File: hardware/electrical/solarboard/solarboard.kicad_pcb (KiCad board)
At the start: 2 copper layers, 10 parts, among them J1 Conn_01x02_Pin

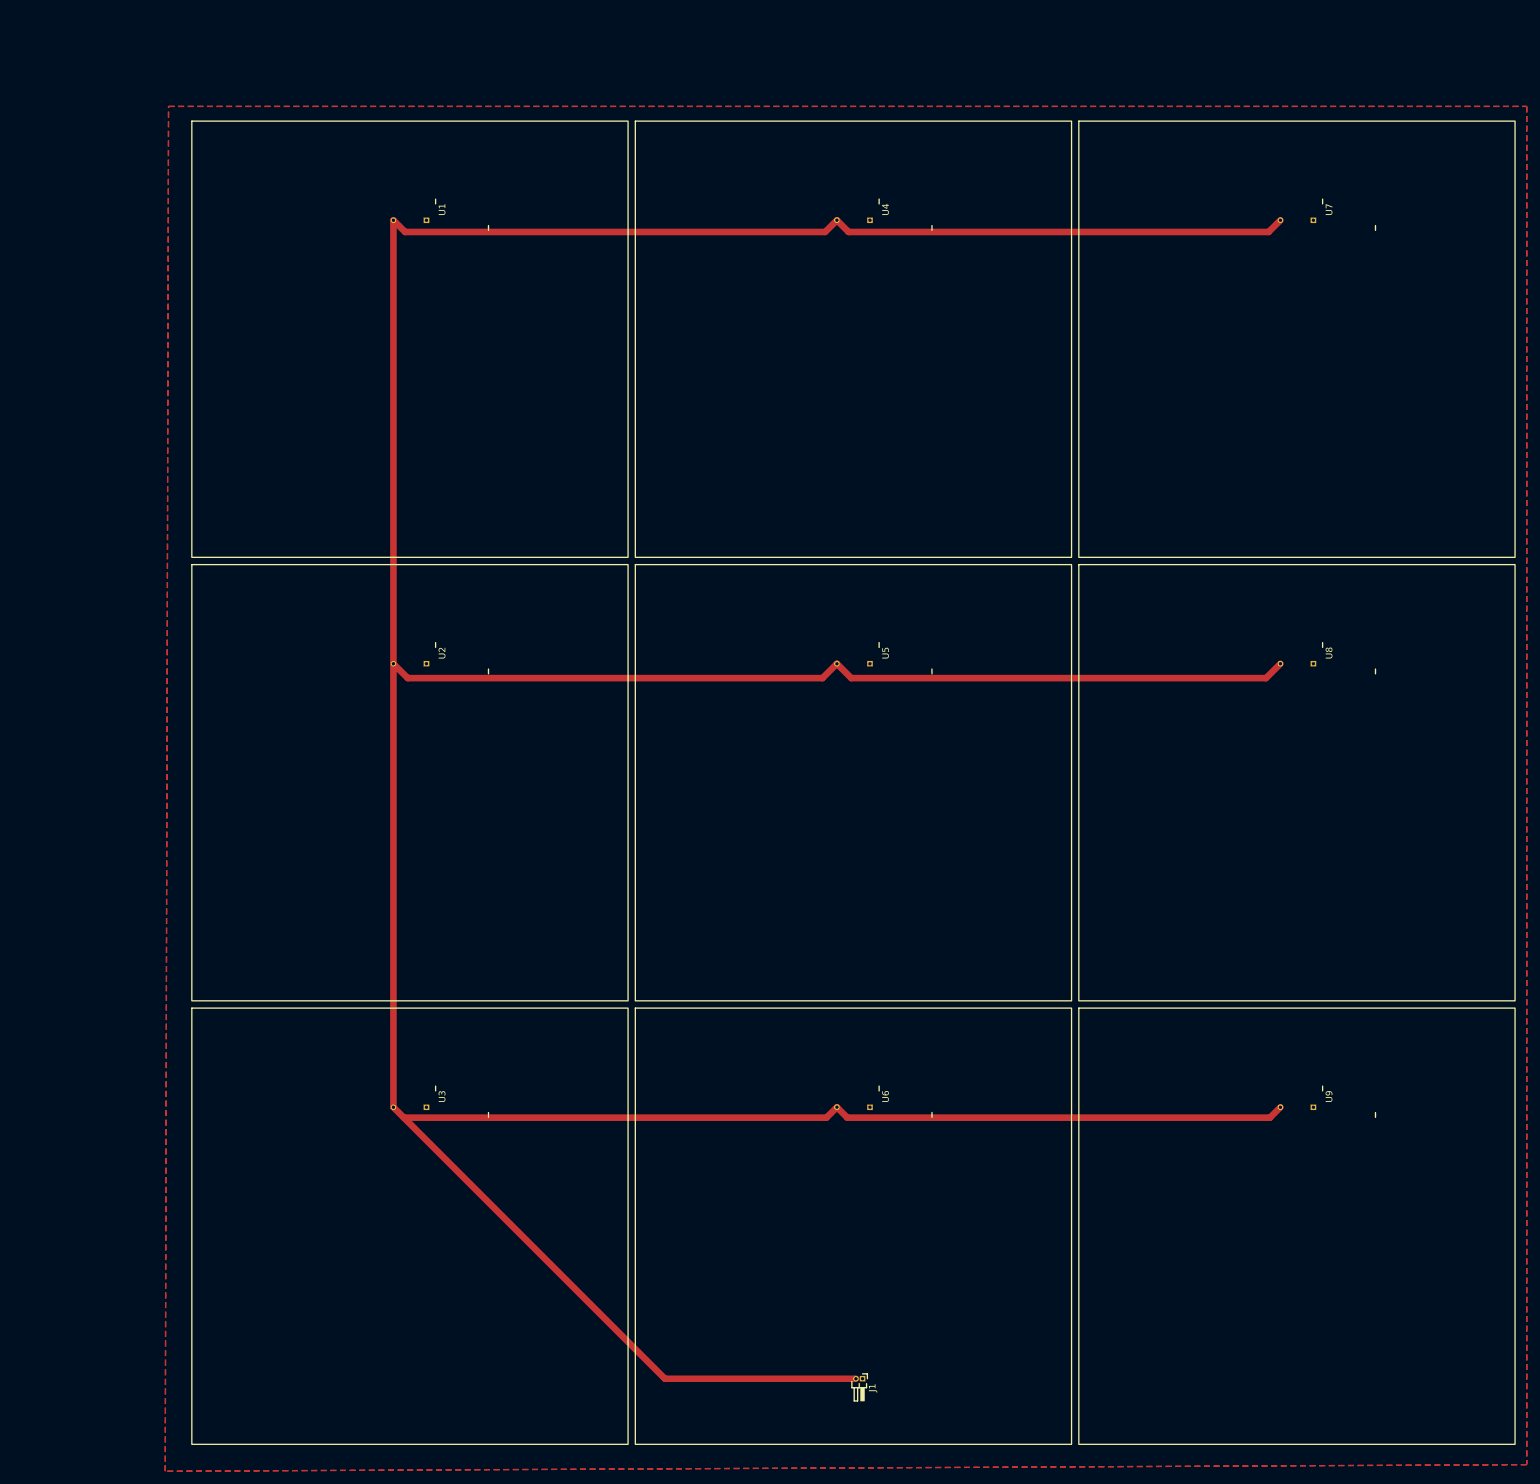
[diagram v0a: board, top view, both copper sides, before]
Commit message: revision solar board
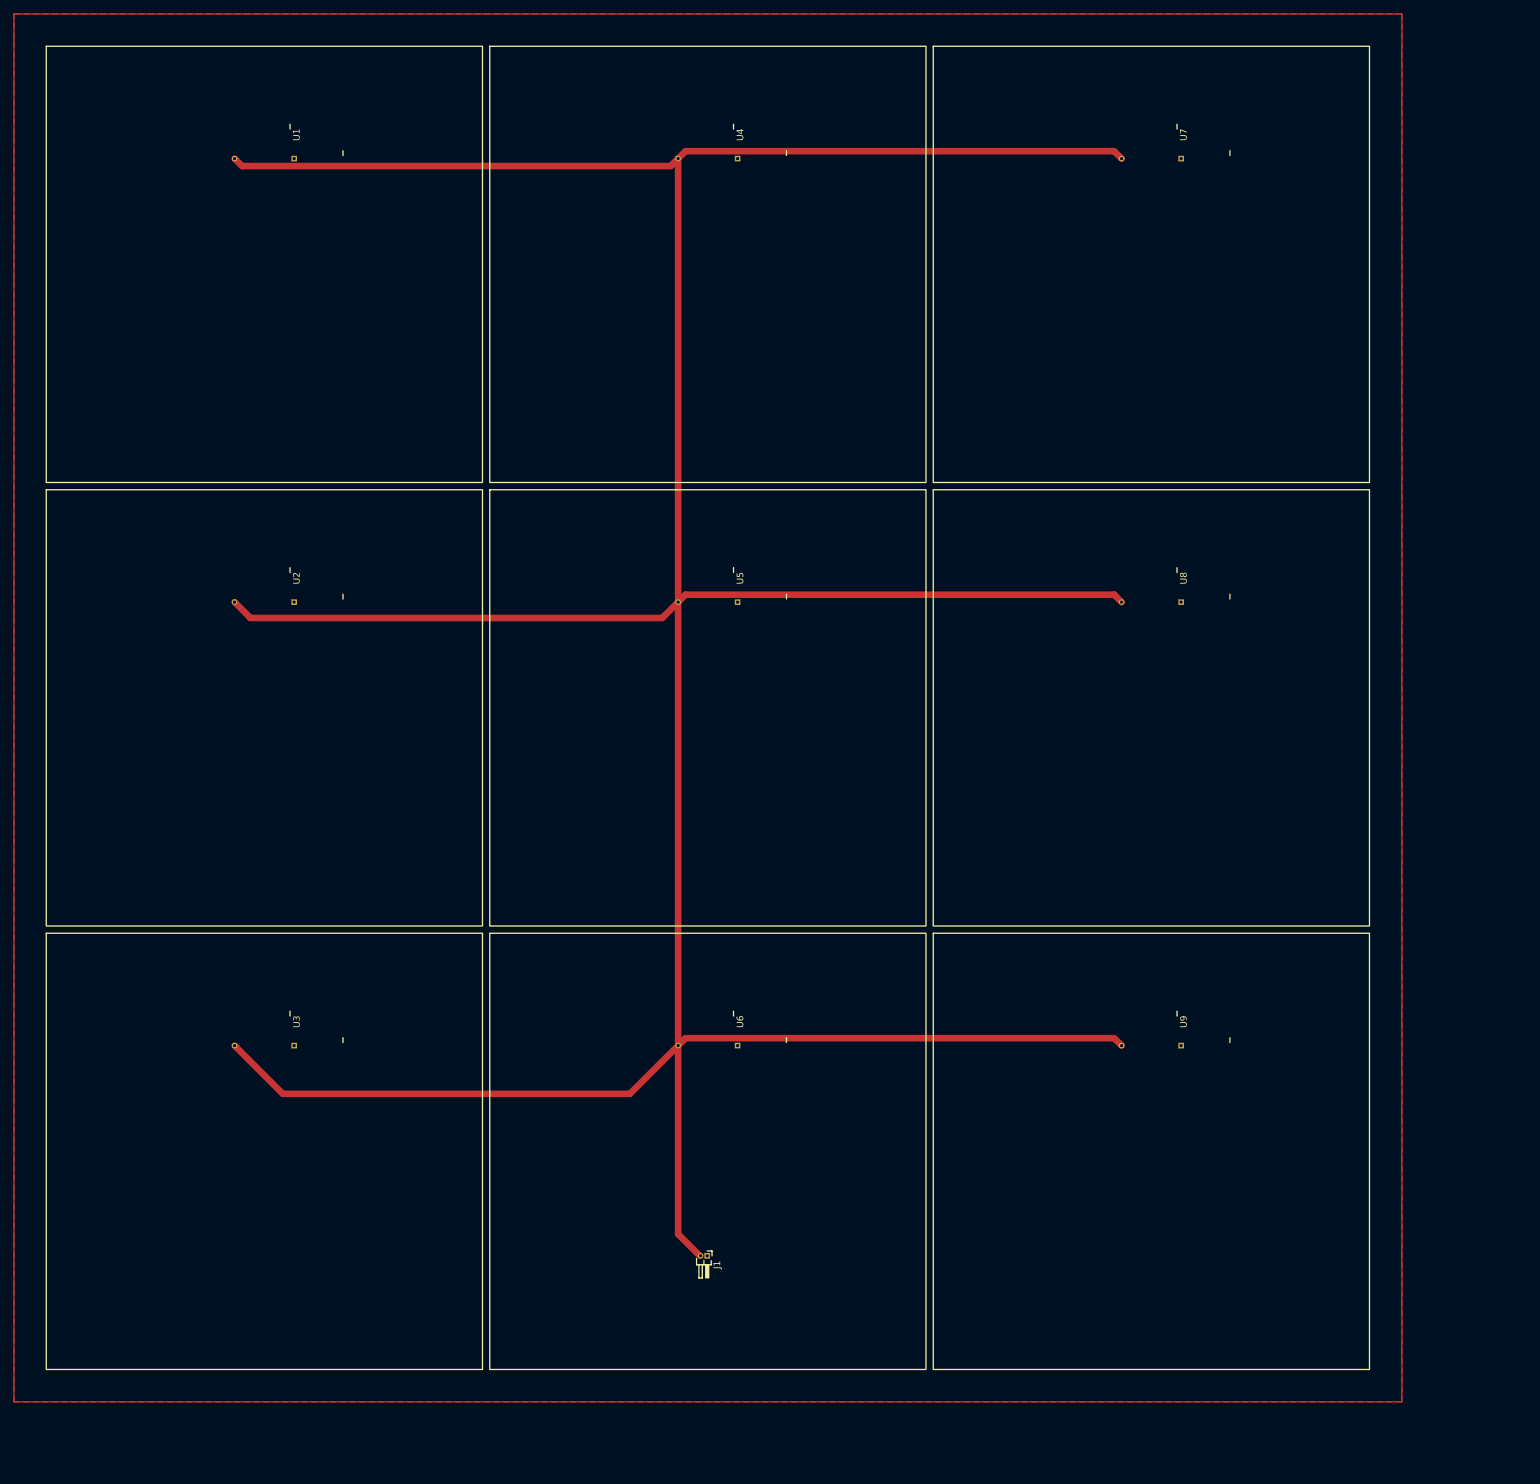
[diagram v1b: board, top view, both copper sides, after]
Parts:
- moved J1 30.0 mm to (107.0, 175.9)
- moved U3 24.8 mm to (40.0, 142.1)
- moved U6 24.8 mm to (107.1, 142.1)
- moved U9 24.8 mm to (174.2, 142.1)
- moved U4 24.8 mm to (107.1, 7.90)
- moved U5 24.8 mm to (107.1, 75.0)
- moved U7 24.8 mm to (174.2, 7.90)
- moved U8 24.8 mm to (174.2, 75.0)
- moved U1 24.8 mm to (40.0, 7.90)
- moved U2 24.8 mm to (40.0, 75.0)
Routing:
- net Net-(J1-Pin_2): track 632.9 -> 581.7 mm
- removed copper zone on F.Cu, net (none)
